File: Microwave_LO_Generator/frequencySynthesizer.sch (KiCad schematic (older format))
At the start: 27 parts, among them J4 Conn_01x05_Male, U1 ADF4150HV, X1 IQXT-220-1

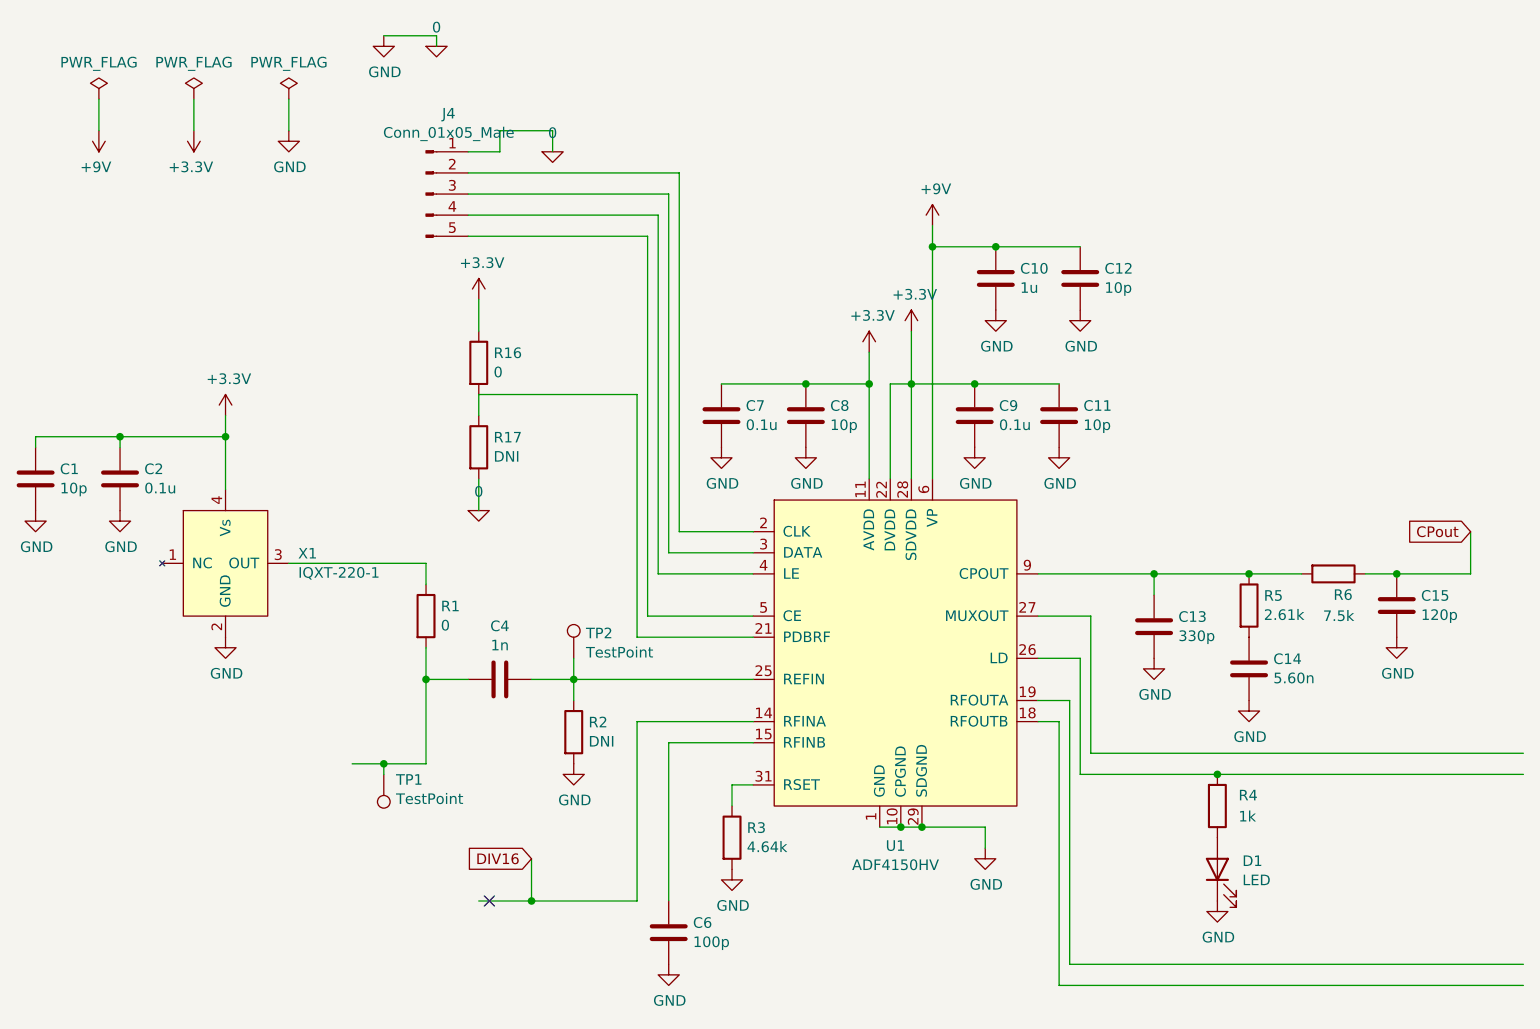
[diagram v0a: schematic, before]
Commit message: A lot of change
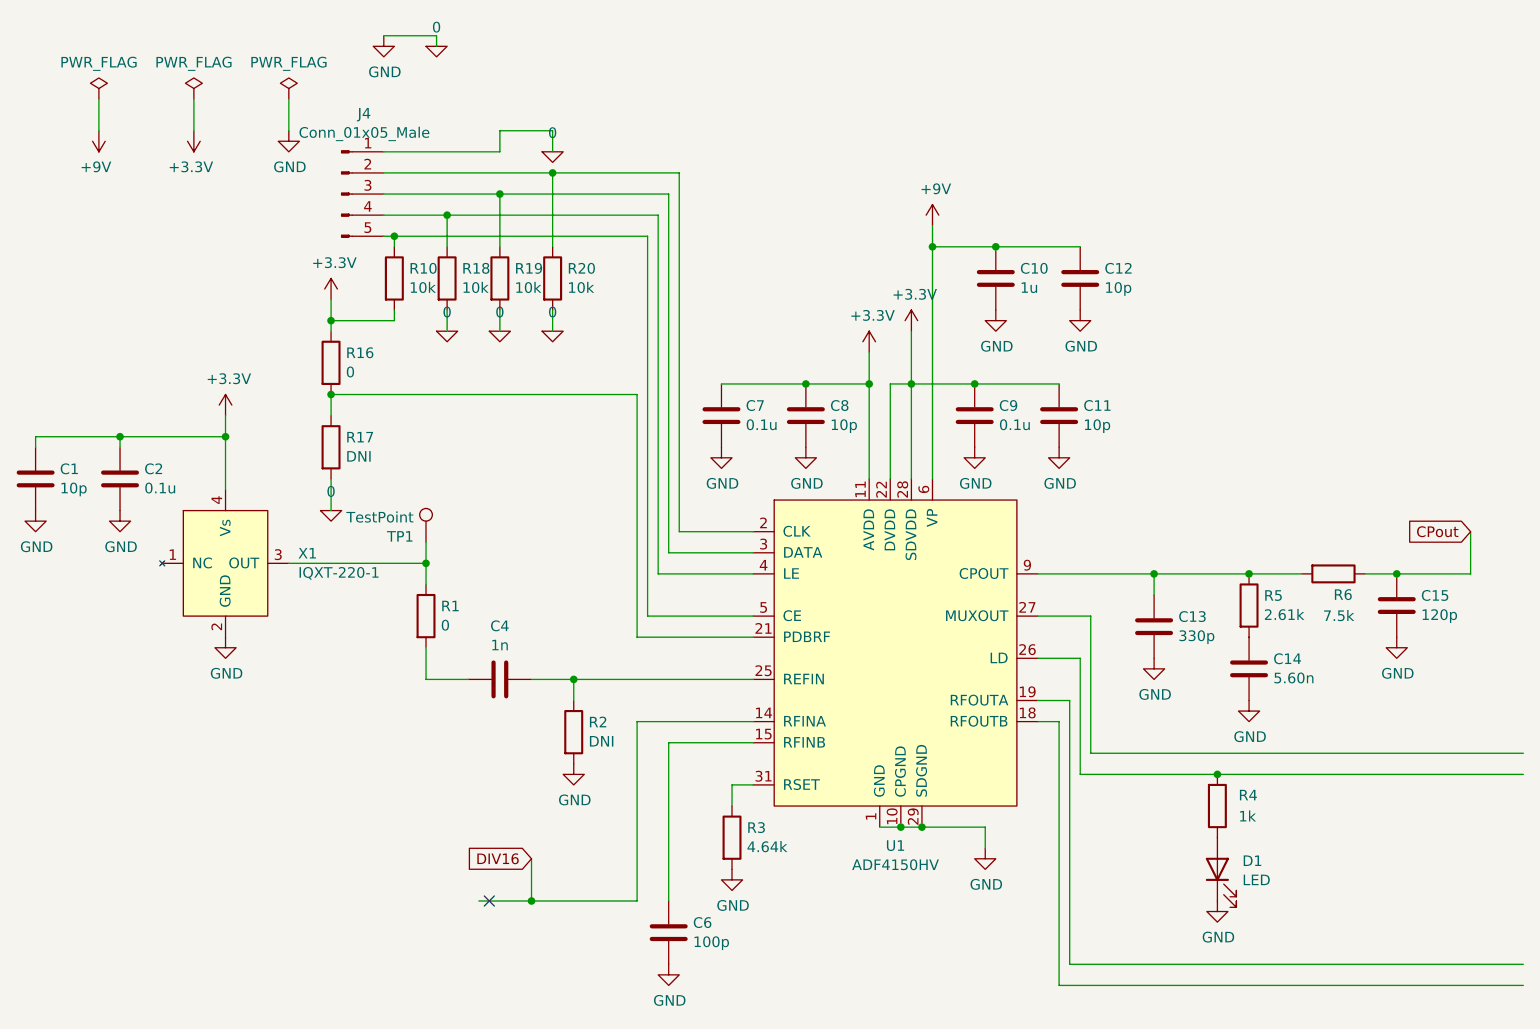
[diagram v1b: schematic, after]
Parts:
- removed TP2: TestPoint, TestPoint:TestPoint_Loop_D2.60mm_Drill1.6mm_Beaded, symbol frequencySynthesizer-rescue:TestPoint-frequencySintesizer
- added R10, R18, R19, R20: 10k, Resistor_SMD:R_0402_1005Metric_Pad0.72x0.64mm_HandSolder, symbol Device:R
- U1: footprint Package_CSP:LFCSP-32-1EP_5x5mm_P0.5mm_EP3.25x3.25mm -> Microwave_LO_Generator:LFCSP-32-1EP_5x5mm_P0.5mm_mod
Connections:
- wire segments 92 -> 102
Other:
- moved on the sheet: J4, R16, R17, TP1
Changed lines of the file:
@@
 Wire Wire Line
 	3150 4100 3350 4100
-Wire Wire Line
-	3150 4100 3150 4500
-Wire Wire Line
-	3150 4500 2950 4500
-Connection ~ 3150 4100
 $Comp
 L Device:R R2
@@
 	3850 4200 3850 4100
 Connection ~ 3850 4100
-Connection ~ 2950 4500
-Wire Wire Line
-	2950 4500 2800 4500
-Wire Wire Line
-	2950 4500 2950 4550
-$Comp
-L frequencySynthesizer-rescue:TestPoint-frequencySintesizer TP2
-U 1 1 5FBBB2E0
-P 3850 4000
-F 0 "TP2" H 3908 4118 50  0000 L CNN
-F 1 "TestPoint" H 3908 4027 50  0000 L CNN
-F 2 "TestPoint:TestPoint_Loop_D2.60mm_Drill1.6mm_Beaded" H 4050 4000 50  0001 C CNN
-F 3 "https://www.mouser.it/datasheet/2/215/005-5009-741293.pdf" H 4050 4000 50  0001 C CNN
-F 4 "5007" H 3850 4000 50  0001 C CNN "Manufacturer/Part Number"
-F 5 "Mouser 534-5007" H 3850 4000 50  0001 C CNN "Supplier Stock Code"
-	1    3850 4000
-	1    0    0    -1
-$EndComp
 $Comp
 L frequencySynthesizer-rescue:TestPoint-frequencySintesizer TP1
 U 1 1 5FBBC038
-P 2950 4550
-F 0 "TP1" H 2892 4576 50  0000 R CNN
-F 1 "TestPoint" H 2892 4667 50  0000 R CNN
-F 2 "TestPoint:TestPoint_Loop_D2.60mm_Drill1.6mm_Beaded" H 3150 4550 50  0001 C CNN
-F 3 "https://www.mouser.it/datasheet/2/215/005-5009-741293.pdf" H 3150 4550 50  0001 C CNN
-F 4 "5007" H 2950 4550 50  0001 C CNN "Manufacturer/Part Number"
-F 5 "Mouser 534-5007" H 2950 4550 50  0001 C CNN "Supplier Stock Code"
-	1    2950 4550
-	-1   0    0    1
-$EndComp
-Wire Wire Line
-	3850 4100 3850 4000
+P 3150 3450
+F 0 "TP1" H 3092 3476 50  0000 R CNN
+F 1 "TestPoint" H 3092 3567 50  0000 R CNN
+F 2 "TestPoint:TestPoint_Loop_D2.60mm_Drill1.6mm_Beaded" H 3350 3450 50  0001 C CNN
+F 3 "https://www.mouser.it/datasheet/2/215/005-5009-741293.pdf" H 3350 3450 50  0001 C CNN
+F 4 "5007" H 3150 3450 50  0001 C CNN "Manufacturer/Part Number"
+F 5 "Mouser 534-5007" H 3150 3450 50  0001 C CNN "Supplier Stock Code"
+	1    3150 3450
+	1    0    0    -1
+$EndComp
 Wire Wire Line
 	3850 4100 4700 4100
@@
 	4350 3400 4350 1700
 Wire Wire Line
-	4350 1700 3350 1700
-Wire Wire Line
 	4700 3500 4300 3500
 Wire Wire Line
 	4300 3500 4300 1800
 Wire Wire Line
-	4300 1800 3350 1800
-Wire Wire Line
 	4700 3600 4250 3600
 Wire Wire Line
 	4250 3600 4250 1900
 Wire Wire Line
-	4250 1900 3350 1900
-Wire Wire Line
 	4700 3800 4200 3800
 Wire Wire Line
 	4200 3800 4200 2000
-Wire Wire Line
-	4200 2000 3350 2000
 Wire Wire Line
 	4700 3900 4150 3900
@@
 Wire Wire Line
 	5800 4800 5800 4900
-Wire Wire Line
-	3400 2750 4150 2750
 $Comp
 L Device:C C6
@@
 F 0 "U1" H 5375 3111 50  0000 C CNN
 F 1 "ADF4150HV" H 5375 3020 50  0000 C CNN
-F 2 "Package_CSP:LFCSP-32-1EP_5x5mm_P0.5mm_EP3.25x3.25mm" H 5400 4000 50  0001 C CNN
+F 2 "Microwave_LO_Generator:LFCSP-32-1EP_5x5mm_P0.5mm_mod" H 5400 4000 50  0001 C CNN
 F 3 "https://www.analog.com/media/en/technical-documentation/data-sheets/ADF4150HV.pdf" H 5100 4000 50  0001 C CNN
 F 4 "ADF4150HVBCPZ" H 5400 4000 50  0001 C CNN "Manufacturer/Part Number"
@@
 Wire Wire Line
 	3750 1500 3750 1600
-$Comp
-L Connector:Conn_01x05_Male J4
-U 1 1 5FCD328E
-P 3150 1800
-F 0 "J4" H 3258 2181 50  0000 C CNN
-F 1 "Conn_01x05_Male" H 3258 2090 50  0000 C CNN
-F 2 "Connector_PinHeader_2.54mm:PinHeader_1x05_P2.54mm_Vertical" H 3150 1800 50  0001 C CNN
-F 3 "~" H 3150 1800 50  0001 C CNN
-	1    3150 1800
-	1    0    0    -1
-$EndComp
 Wire Wire Line
 	3500 1500 3500 1600
-Wire Wire Line
-	3500 1600 3350 1600
 Wire Wire Line
 	3500 1500 3750 1500
@@
 L Device:R R17
 U 1 1 5FD3B0E5
-P 3400 3000
-F 0 "R17" H 3470 3046 50  0000 L CNN
-F 1 "DNI" H 3470 2955 50  0000 L CNN
-F 2 "Resistor_SMD:R_0603_1608Metric_Pad0.98x0.95mm_HandSolder" V 3330 3000 50  0001 C CNN
-F 3 "~" H 3400 3000 50  0001 C CNN
-F 4 "D/CRCW0402 kit in dipartimento" H 3400 3000 50  0001 C CNN "Supplier Stock Code"
-	1    3400 3000
-	1    0    0    -1
-$EndComp
-Wire Wire Line
-	3400 3150 3400 3300
-Wire Wire Line
-	3400 2750 3400 2850
-$Comp
-L Device:R R16
-U 1 1 5FD46A04
-P 3400 2600
-F 0 "R16" H 3470 2646 50  0000 L CNN
-F 1 "0" H 3470 2555 50  0000 L CNN
-F 2 "Resistor_SMD:R_0402_1005Metric_Pad0.72x0.64mm_HandSolder" V 3330 2600 50  0001 C CNN
-F 3 "~" H 3400 2600 50  0001 C CNN
-F 4 "D/CRCW0402 kit in dipartimento" H 3400 2600 50  0001 C CNN "Supplier Stock Code"
-	1    3400 2600
-	1    0    0    -1
-$EndComp
+P 2700 3000
+F 0 "R17" H 2770 3046 50  0000 L CNN
+F 1 "DNI" H 2770 2955 50  0000 L CNN
+F 2 "Resistor_SMD:R_0603_1608Metric_Pad0.98x0.95mm_HandSolder" V 2630 3000 50  0001 C CNN
+F 3 "~" H 2700 3000 50  0001 C CNN
+F 4 "D/CRCW0402 kit in dipartimento" H 2700 3000 50  0001 C CNN "Supplier Stock Code"
+	1    2700 3000
+	1    0    0    -1
+$EndComp
+Wire Wire Line
+	2700 3150 2700 3300
+Wire Wire Line
+	2700 2750 2700 2850
 $Comp
 L pspice:0 #GND0123
 U 1 1 5FD49CF4
-P 3400 3300
-F 0 "#GND0123" H 3400 3200 50  0001 C CNN
-F 1 "0" H 3400 3389 50  0000 C CNN
-F 2 "" H 3400 3300 50  0001 C CNN
-F 3 "~" H 3400 3300 50  0001 C CNN
-	1    3400 3300
+P 2700 3300
+F 0 "#GND0123" H 2700 3200 50  0001 C CNN
+F 1 "0" H 2700 3389 50  0000 C CNN
+F 2 "" H 2700 3300 50  0001 C CNN
+F 3 "~" H 2700 3300 50  0001 C CNN
+	1    2700 3300
 	1    0    0    -1
 $EndComp
@@
 	1    0    0    -1
 $EndComp
+Wire Wire Line
+	2700 2300 2700 2400
 $Comp
 L power:+3.3V #PWR0138
 U 1 1 5FD4CD79
-P 3400 2300
-F 0 "#PWR0138" H 3400 2150 50  0001 C CNN
-F 1 "+3.3V" H 3415 2473 50  0000 C CNN
-F 2 "" H 3400 2300 50  0001 C CNN
-F 3 "" H 3400 2300 50  0001 C CNN
-	1    3400 2300
-	1    0    0    -1
-$EndComp
-Wire Wire Line
-	3400 2300 3400 2450
+P 2700 2300
+F 0 "#PWR0138" H 2700 2150 50  0001 C CNN
+F 1 "+3.3V" H 2715 2473 50  0000 C CNN
+F 2 "" H 2700 2300 50  0001 C CNN
+F 3 "" H 2700 2300 50  0001 C CNN
+	1    2700 2300
+	1    0    0    -1
+$EndComp
+$Comp
+L Device:R R16
+U 1 1 5FD46A04
+P 2700 2600
+F 0 "R16" H 2770 2646 50  0000 L CNN
+F 1 "0" H 2770 2555 50  0000 L CNN
+F 2 "Resistor_SMD:R_0402_1005Metric_Pad0.72x0.64mm_HandSolder" V 2630 2600 50  0001 C CNN
+F 3 "~" H 2700 2600 50  0001 C CNN
+F 4 "D/CRCW0402 kit in dipartimento" H 2700 2600 50  0001 C CNN "Supplier Stock Code"
+	1    2700 2600
+	1    0    0    -1
+$EndComp
+$Comp
+L Connector:Conn_01x05_Male J4
+U 1 1 5FCD328E
+P 2750 1800
+F 0 "J4" H 2858 2181 50  0000 C CNN
+F 1 "Conn_01x05_Male" H 2858 2090 50  0000 C CNN
+F 2 "Connector_PinHeader_2.54mm:PinHeader_1x05_P2.54mm_Vertical" H 2750 1800 50  0001 C CNN
+F 3 "~" H 2750 1800 50  0001 C CNN
+	1    2750 1800
+	1    0    0    -1
+$EndComp
+$Comp
+L Device:R R10
+U 1 1 5FCB72FC
+P 3000 2200
+F 0 "R10" H 3070 2246 50  0000 L CNN
+F 1 "10k" H 3070 2155 50  0000 L CNN
+F 2 "Resistor_SMD:R_0402_1005Metric_Pad0.72x0.64mm_HandSolder" V 2930 2200 50  0001 C CNN
+F 3 "~" H 3000 2200 50  0001 C CNN
+F 4 "D/CRCW0402 kit in dipartimento" H 3000 2200 50  0001 C CNN "Supplier Stock Code"
+	1    3000 2200
+	1    0    0    -1
+$EndComp
+Connection ~ 2700 2750
+Wire Wire Line
+	3000 2050 3000 2000
+Wire Wire Line
+	3000 2350 3000 2400
+Wire Wire Line
+	3000 2400 2700 2400
+Connection ~ 2700 2400
+Wire Wire Line
+	2700 2400 2700 2450
+$Comp
+L Device:R R18
+U 1 1 5FCC84F5
+P 3250 2200
+F 0 "R18" H 3320 2246 50  0000 L CNN
+F 1 "10k" H 3320 2155 50  0000 L CNN
+F 2 "Resistor_SMD:R_0402_1005Metric_Pad0.72x0.64mm_HandSolder" V 3180 2200 50  0001 C CNN
+F 3 "~" H 3250 2200 50  0001 C CNN
+F 4 "D/CRCW0402 kit in dipartimento" H 3250 2200 50  0001 C CNN "Supplier Stock Code"
+	1    3250 2200
+	1    0    0    -1
+$EndComp
+$Comp
+L Device:R R19
+U 1 1 5FCCB177
+P 3500 2200
+F 0 "R19" H 3570 2246 50  0000 L CNN
+F 1 "10k" H 3570 2155 50  0000 L CNN
+F 2 "Resistor_SMD:R_0402_1005Metric_Pad0.72x0.64mm_HandSolder" V 3430 2200 50  0001 C CNN
+F 3 "~" H 3500 2200 50  0001 C CNN
+F 4 "D/CRCW0402 kit in dipartimento" H 3500 2200 50  0001 C CNN "Supplier Stock Code"
+	1    3500 2200
+	1    0    0    -1
+$EndComp
+$Comp
+L Device:R R20
+U 1 1 5FCCDA73
+P 3750 2200
+F 0 "R20" H 3820 2246 50  0000 L CNN
+F 1 "10k" H 3820 2155 50  0000 L CNN
+F 2 "Resistor_SMD:R_0402_1005Metric_Pad0.72x0.64mm_HandSolder" V 3680 2200 50  0001 C CNN
+F 3 "~" H 3750 2200 50  0001 C CNN
+F 4 "D/CRCW0402 kit in dipartimento" H 3750 2200 50  0001 C CNN "Supplier Stock Code"
+	1    3750 2200
+	1    0    0    -1
+$EndComp
+Wire Wire Line
+	3250 2050 3250 1900
+Wire Wire Line
+	3500 2050 3500 1800
+Wire Wire Line
+	2700 2750 4150 2750
+Wire Wire Line
+	2950 1600 3500 1600
+Wire Wire Line
+	2950 1700 3750 1700
+Wire Wire Line
+	2950 1800 3500 1800
+Wire Wire Line
+	2950 1900 3250 1900
+Wire Wire Line
+	2950 2000 3000 2000
+Connection ~ 3250 1900
+Wire Wire Line
+	3250 1900 4250 1900
+Connection ~ 3500 1800
+Connection ~ 3000 2000
+Wire Wire Line
+	3000 2000 4200 2000
+Wire Wire Line
+	3500 1800 4300 1800
+Wire Wire Line
+	3750 2050 3750 1700
+Connection ~ 3750 1700
+Wire Wire Line
+	3750 1700 4350 1700
+$Comp
+L pspice:0 #GND0130
+U 1 1 5FD1A641
+P 3250 2450
+F 0 "#GND0130" H 3250 2350 50  0001 C CNN
+F 1 "0" H 3250 2539 50  0000 C CNN
+F 2 "" H 3250 2450 50  0001 C CNN
+F 3 "~" H 3250 2450 50  0001 C CNN
+	1    3250 2450
+	1    0    0    -1
+$EndComp
+$Comp
+L pspice:0 #GND0131
+U 1 1 5FD1AD97
+P 3500 2450
+F 0 "#GND0131" H 3500 2350 50  0001 C CNN
+F 1 "0" H 3500 2539 50  0000 C CNN
+F 2 "" H 3500 2450 50  0001 C CNN
+F 3 "~" H 3500 2450 50  0001 C CNN
+	1    3500 2450
+	1    0    0    -1
+$EndComp
+$Comp
+L pspice:0 #GND0132
+U 1 1 5FD1AF60
+P 3750 2450
+F 0 "#GND0132" H 3750 2350 50  0001 C CNN
+F 1 "0" H 3750 2539 50  0000 C CNN
+F 2 "" H 3750 2450 50  0001 C CNN
+F 3 "~" H 3750 2450 50  0001 C CNN
+	1    3750 2450
+	1    0    0    -1
+$EndComp
+Wire Wire Line
+	3250 2450 3250 2350
+Wire Wire Line
+	3500 2450 3500 2350
+Wire Wire Line
+	3750 2450 3750 2350
+Wire Wire Line
+	3150 3450 3150 3550
+Connection ~ 3150 3550
 $EndSCHEMATC
